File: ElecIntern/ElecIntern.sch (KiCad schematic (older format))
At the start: 19 parts, among them J1 Conn_01x02, J2 Conn_Servo, J3 Conn_01x05, J4 Conn_01x05, U1 MR45V200B, U3 PMOS, U4 R-78C5.0-1.0, U5 R-78C3.3-1.0, U7 TEENSY3.2, U8 Xbee802.15.4, U9 MPU-6050

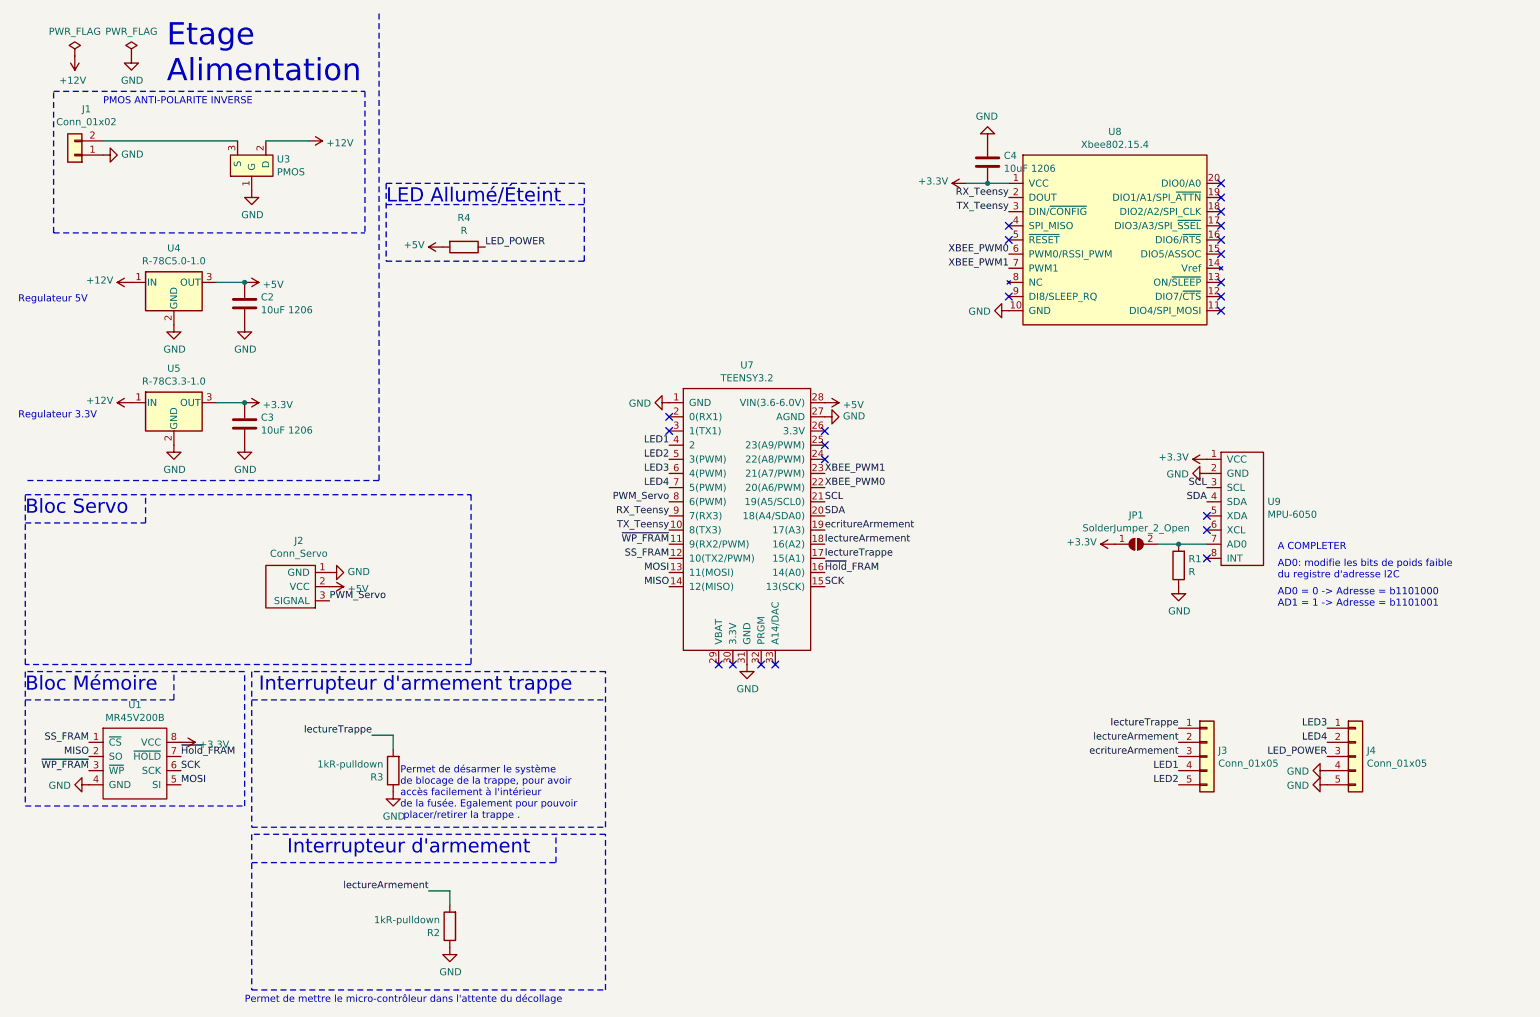
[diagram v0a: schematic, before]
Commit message: Grosse mise à jour
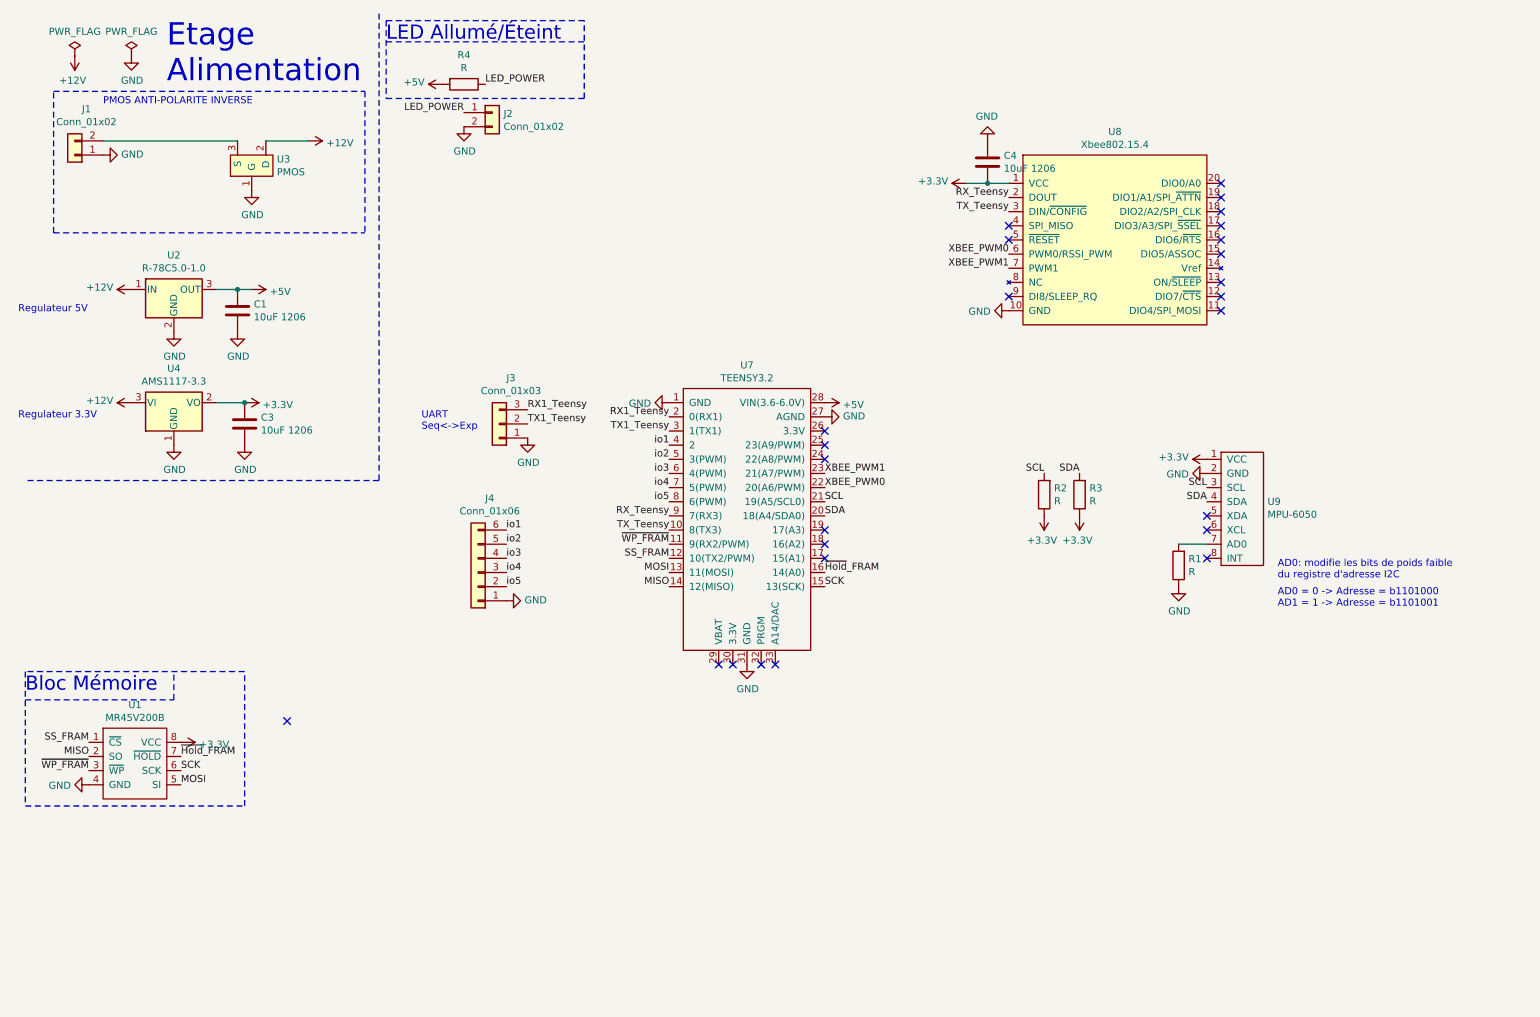
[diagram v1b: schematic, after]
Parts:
- removed C2: 10uF 1206, Capacitor_SMD:C_1206_3216Metric_Pad1.42x1.75mm_HandSolder, symbol Device:C
- removed J2: Conn_Servo, Connector_JST:JST_XH_B3B-XH-A_1x03_P2.50mm_Vertical, symbol PI06:Conn_Servo
- removed J3, J4: Conn_01x05, Connector_JST:JST_XH_B5B-XH-A_1x05_P2.50mm_Vertical, symbol Connector_Generic:Conn_01x05
- removed JP1: SolderJumper_2_Open, Resistor_SMD:R_1206_3216Metric_Pad1.42x1.75mm_HandSolder, symbol Jumper:SolderJumper_2_Open
- removed U4: R-78C5.0-1.0, Converter_DCDC:Converter_DCDC_RECOM_R-78E-0.5_THT, symbol Regulator_Switching:R-78C5.0-1.0
- removed U5: R-78C3.3-1.0, Converter_DCDC:Converter_DCDC_RECOM_R-78E-0.5_THT, symbol Regulator_Switching:R-78C3.3-1.0
- added C1: 10uF 1206, Capacitor_SMD:C_1206_3216Metric_Pad1.42x1.75mm_HandSolder, symbol Device:C
- added J2: Conn_01x02, Connector_JST:JST_XH_B2B-XH-A_1x02_P2.50mm_Vertical, symbol Connector_Generic:Conn_01x02
- added J3: Conn_01x03, Connector_JST:JST_XH_B3B-XH-AM_1x03_P2.50mm_Vertical, symbol Connector_Generic:Conn_01x03
- added J4: Conn_01x06, Connector_JST:JST_XH_B6B-XH-AM_1x06_P2.50mm_Vertical, symbol Connector_Generic:Conn_01x06
- added U2: R-78C5.0-1.0, Converter_DCDC:Converter_DCDC_RECOM_R-78E-0.5_THT, symbol Regulator_Switching:R-78C5.0-1.0
- added U4: AMS1117-3.3, Package_TO_SOT_SMD:SOT-223-3_TabPin2, symbol Regulator_Linear:AMS1117-3.3
- J1: footprint rex:BatConn -> Connector_JST:JST_XH_B2B-XH-AM_1x02_P2.50mm_Vertical
- R2, R3: value 1kR-pulldown -> R
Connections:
- net +12V: now also U2.1 (IN), U4.3 (VI)
- net +3V3: now also R2.1, R3.1, U4.2 (VO)
- net +5V: now also C1.1, U2.3 (OUT)
- net GND: now also C1.2, J2.2 (Pin_2), J3.1 (Pin_1), J4.1 (Pin_1), U2.2 (GND), U4.1 (GND); no longer R2.1, R3.1
- net LED_POWER: now also J2.1 (Pin_1)
- net SCL: now also R2.2
- net SDA: now also R3.2
- net RX1_Teensy: now reaches U7.2 (0(RX1))
- net RX1_Teensy: now also J3.3 (Pin_3)
- net TX1_Teensy: now reaches U7.3 (1(TX1))
- net TX1_Teensy: now also J3.2 (Pin_2)
- net LED1 renamed io1
- net io1: now also J4.6 (Pin_6)
- net LED2 renamed io2
- net io2: now also J4.5 (Pin_5)
- net LED3 renamed io3
- net io3: now also J4.4 (Pin_4)
- net LED4 renamed io4
- net io4: now also J4.3 (Pin_3)
- net PWM_Servo renamed io5
- net io5: now also J4.2 (Pin_2)
- net ecritureArmement: no longer names the net of U7.19 (17(A3))
- net lectureArmement: no longer names the net of U7.18 (16(A2))
- net lectureArmement: no longer R2.2
- net lectureTrappe: no longer names the net of U7.17 (15(A1))
- net lectureTrappe: no longer R3.2
- no-connect marks 24 -> 26
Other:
- note added: "Regulateur 5V\n\n"
- note added: "UART\nSeq<->Exp"
- note removed: "A COMPLETER\n"
- note removed: "Bloc Servo"
- note removed: "Interrupteur d'armement"
- note removed: "Interrupteur d'armement trappe"
- note removed: "Permet de désarmer le système \nde blocage de la trappe, pour avoir \naccès facilement à l'intérieur \nde la fusée. Egalement pour pouvoir\n placer/retirer la trappe ."
- note removed: "Permet de mettre le micro-contrôleur dans l'attente du décollage"
- note removed: "Regulateur 5V\n"
- moved on the sheet: R4
